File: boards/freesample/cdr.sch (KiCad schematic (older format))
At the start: 76 parts, among them J6 XILINX_JTAG, U13 SIP32408, U5 TLK10232, U6 LMK61PD0A2

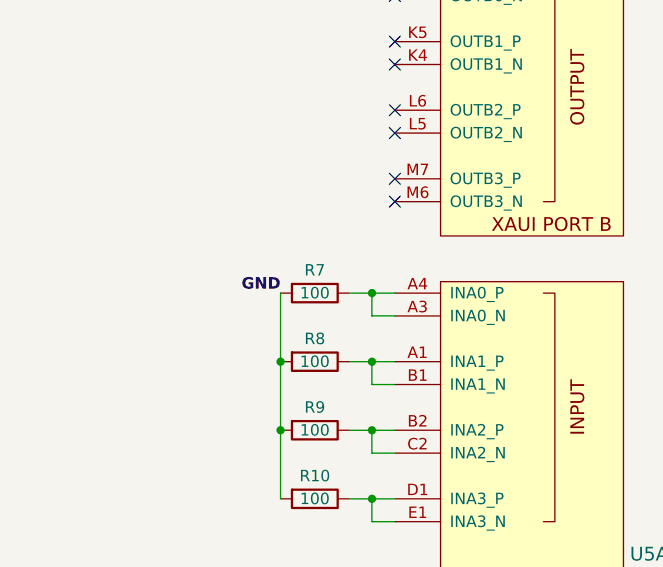
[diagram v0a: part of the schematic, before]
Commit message: Finished initial layout of CDR subsystem
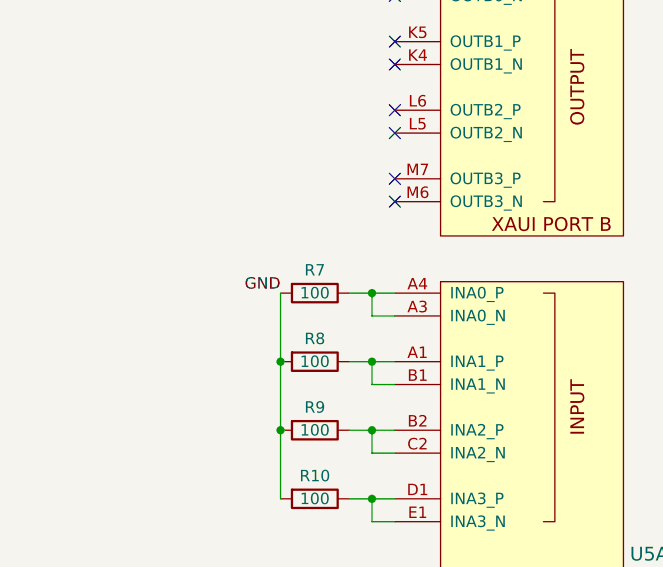
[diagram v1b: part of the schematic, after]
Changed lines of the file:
@@
 Wire Wire Line
 	1650 5800 1650 5500
-Text Label 1650 5200 2    50   ~ 10
+Text Label 1650 5200 2    50   ~ 0
 GND
 NoConn ~ 2150 6500
